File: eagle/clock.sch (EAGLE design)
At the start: 55 parts, among them CN1 ARDUINO_SHIELDNO_SILK, IC1 TPS55330TRE, IC2 TCS3472FN, Q1 BC817-40SMD, Q2 SUD50P04-13L

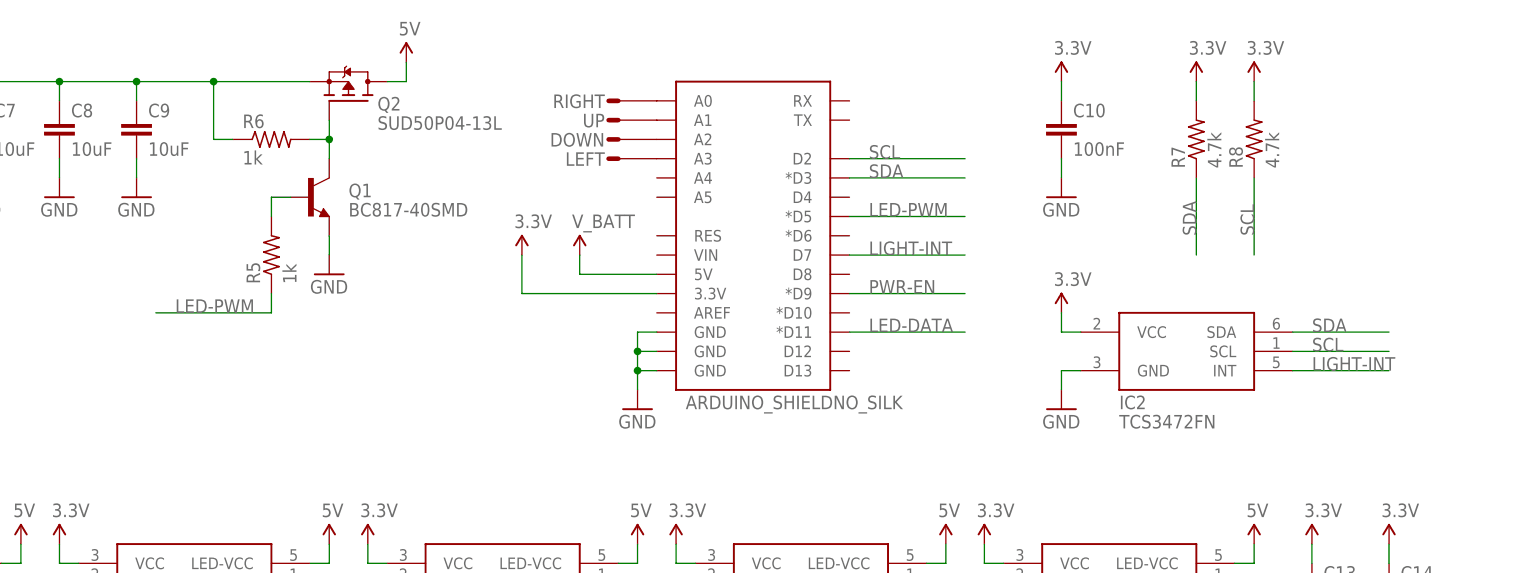
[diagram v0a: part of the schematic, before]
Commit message: Almost finished layout
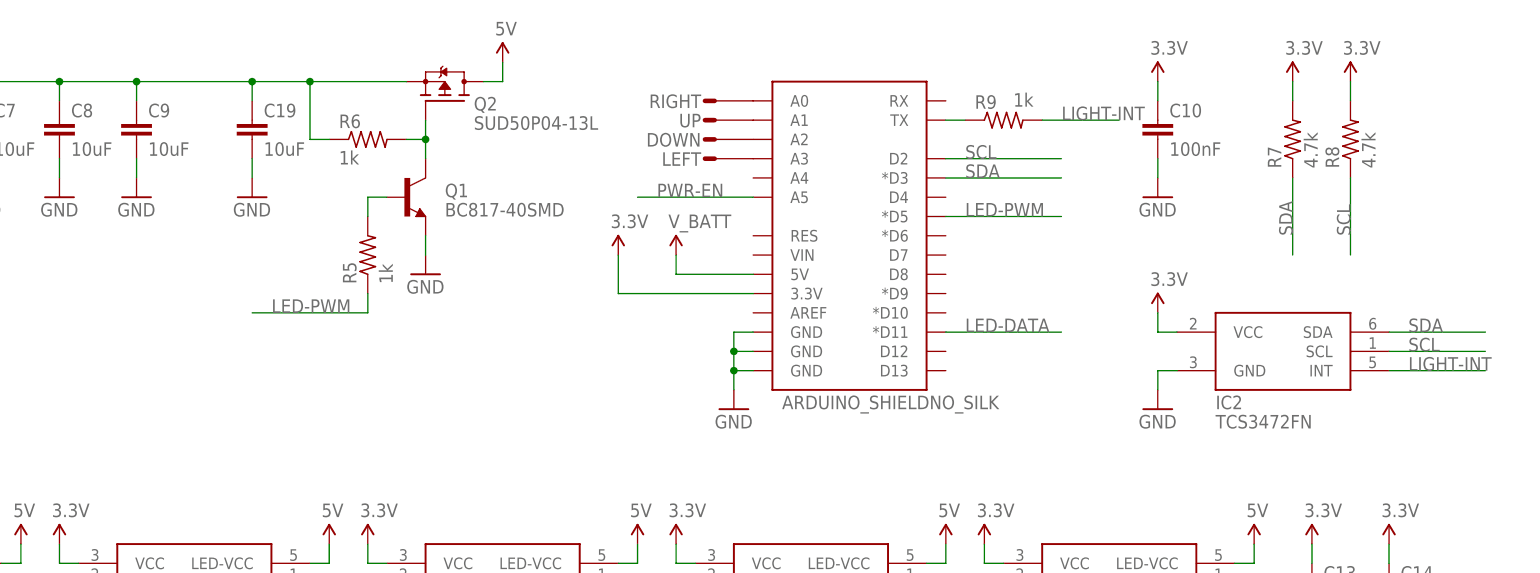
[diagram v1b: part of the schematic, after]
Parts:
- added C19: 10uF, rcl:C-EUC1206K
- added R9: 1k, rcl:R-US_R0603
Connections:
- new net N$6: CN1.TX, R9.1
- net GND: now also C19.2
- net LIGHT-INT: now also R9.2; no longer CN1.D7
- net PWR-EN: now also CN1.A5; no longer CN1.*D9
- net SMPSU-OUTPUT: now also C19.1
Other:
- moved on the sheet: C10, DOWN, IC2, LEFT, Q1, Q2, R5, R6, R7, R8, RIGHT, UP
